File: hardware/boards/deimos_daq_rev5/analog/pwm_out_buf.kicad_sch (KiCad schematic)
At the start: 3 parts

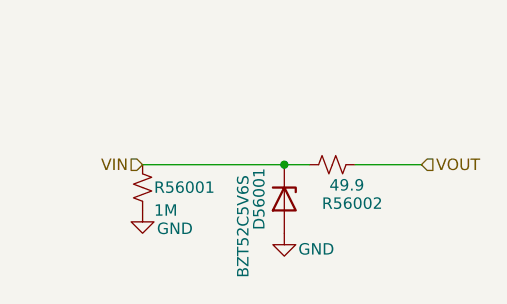
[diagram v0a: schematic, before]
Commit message: restore rev5 and make this rev rev6
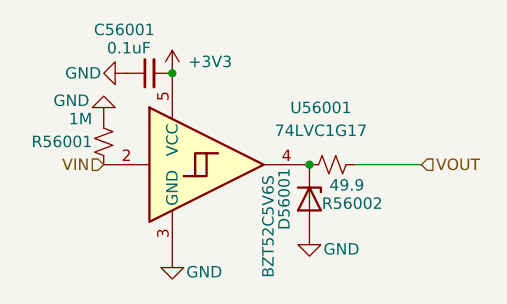
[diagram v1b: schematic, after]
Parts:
- added C56001: 0.1uF, Capacitor_SMD:C_0402_1005Metric, symbol Device:C_Small
- added U56001: 74LVC1G17, Package_TO_SOT_SMD:SOT-23-5, symbol 74xGxx:74LVC1G17
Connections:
- net GND: now also C56001.1, U56001.3 (GND)
- net VIN: now also U56001.2; no longer D56001.1 (K), R56002.1
- new net: D56001.1 (K), R56002.1, U56001.4
- new net +3V3: C56001.2, U56001.5 (VCC)
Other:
- moved on the sheet: D56001, R56001
